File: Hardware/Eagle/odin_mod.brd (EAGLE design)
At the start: 21.4 x 22.8 mm, 36 parts

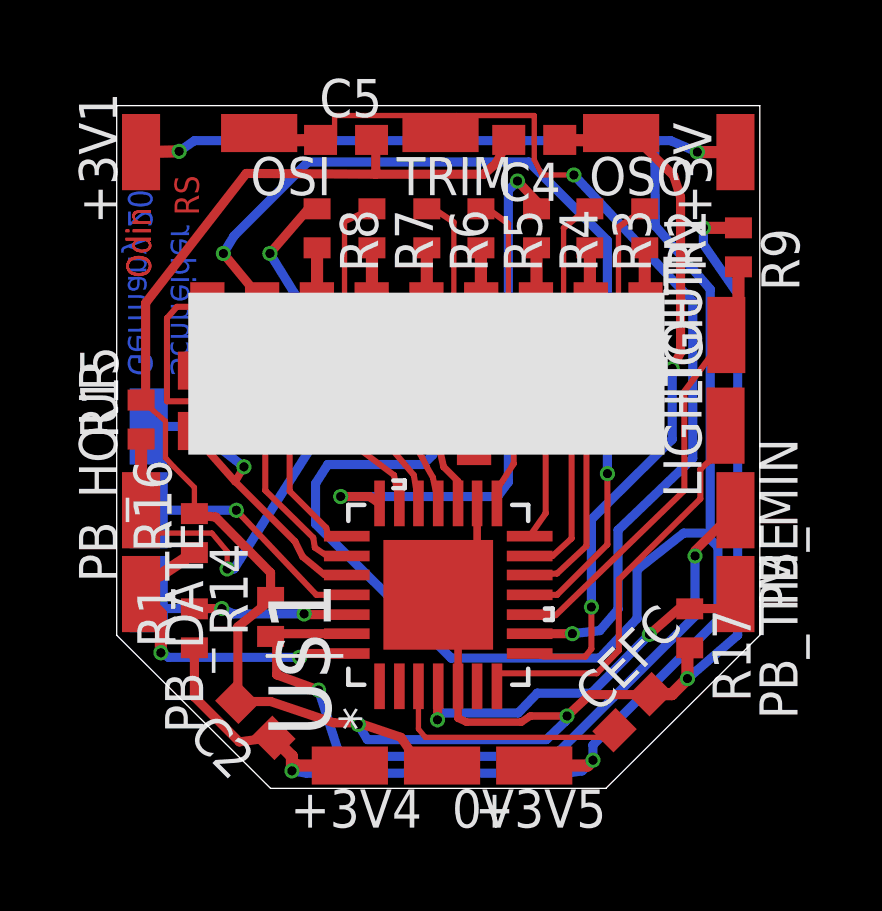
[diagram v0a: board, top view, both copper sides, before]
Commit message: Reviewed Odin module.
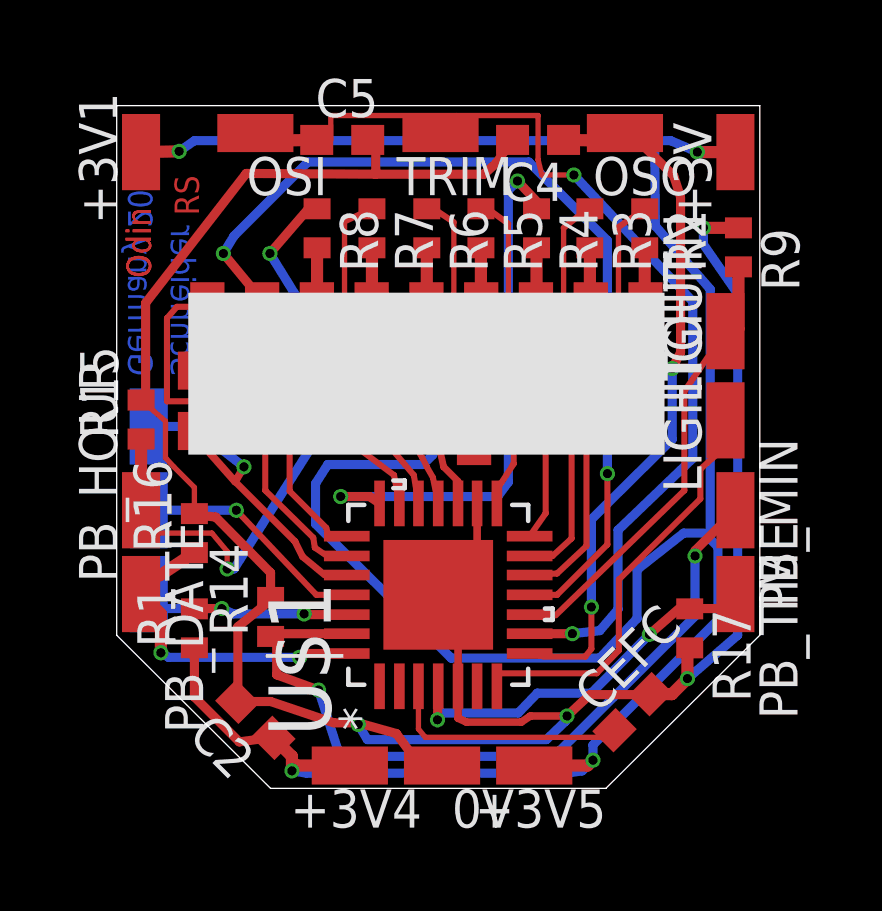
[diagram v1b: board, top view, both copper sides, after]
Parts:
- moved LIGHTOUT 0.18 mm to (20.2, 12.3)
- moved LIGHTIN 0.13 mm to (20.2, 15.2)
- moved C4 0.13 mm to (14.0, 21.6)
- moved C5 0.13 mm to (7.47, 21.6)
- moved OSI 0.13 mm to (4.57, 21.8)
- moved OSO 0.13 mm to (16.9, 21.8)
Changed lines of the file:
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@@
 <element name="R14" library="resistor" package="R0402" value="4.7k" x="5.08" y="5.715" rot="R90"/>
 <element name="R15" library="resistor" package="R0402" value="4.7k" x="0.762" y="12.2936" rot="R90"/>
-<element name="C4" library="resistor" package="C0603" value="12 pF" x="13.8684" y="21.6154" rot="R180"/>
-<element name="C5" library="resistor" package="C0603" value="12 pF" x="7.5946" y="21.6154"/>
+<element name="C4" library="resistor" package="C0603" value="12 pF" x="13.9954" y="21.6154" rot="R180"/>
+<element name="C5" library="resistor" package="C0603" value="12 pF" x="7.4676" y="21.6154"/>
 <element name="U$3" library="pulsar_p3_display" package="PULSAR_P3_LED_DISPLAY" value="PULSAR_P3_DISPLAY" x="2.3368" y="11.1252"/>
 <element name="+3V" library="wirepad" package="SMD1,27-2,54" value="2" x="20.574" y="21.209"/>
@@
 <element name="PAD2" library="wirepad" package="SMD1,27-2,54" value="1" x="1.016" y="9.271" rot="MR0"/>
 <element name="PAD5" library="wirepad" package="SMD1,27-2,54" value="1" x="1.016" y="6.477" rot="MR0"/>
-<element name="OSI" library="wirepad" package="SMD1,27-2,54" value="1" x="4.699" y="21.844" rot="R90"/>
-<element name="OSO" library="wirepad" package="SMD1,27-2,54" value="1" x="16.764" y="21.844" rot="R90"/>
+<element name="OSI" library="wirepad" package="SMD1,27-2,54" value="1" x="4.572" y="21.844" rot="R90"/>
+<element name="OSO" library="wirepad" package="SMD1,27-2,54" value="1" x="16.891" y="21.844" rot="R90"/>
 <element name="+3V4" library="wirepad" package="SMD1,27-2,54" value="1" x="7.7216" y="0.762" rot="R90"/>
 <element name="+3V5" library="wirepad" package="SMD1,27-2,54" value="1" x="13.8684" y="0.762" rot="R90"/>
-<element name="LIGHTIN" library="wirepad" package="SMD1,27-2,54" value="1" x="20.2692" y="15.113"/>
-<element name="LIGHTOUT" library="wirepad" package="SMD1,27-2,54" value="1" x="20.2438" y="12.0904"/>
+<element name="LIGHTIN" library="wirepad" package="SMD1,27-2,54" value="1" x="20.2438" y="15.24"/>
+<element name="LIGHTOUT" library="wirepad" package="SMD1,27-2,54" value="1" x="20.2438" y="12.2682"/>
 <element name="TRIM" library="wirepad" package="SMD1,27-2,54" value="1" x="10.7442" y="21.844" rot="R90"/>
 <element name="R9" library="resistor" package="R0402" value="47k" x="20.6756" y="18.034" rot="R270"/>
@@
 <wire x1="4.2672" y1="20.4978" x2="8.5852" y2="20.4724" width="0.3048" layer="1"/>
 <wire x1="0.9144" y1="13.0302" x2="0.9144" y2="16.1798" width="0.3048" layer="1"/>
-<wire x1="8.7884" y1="21.5646" x2="8.4446" y2="21.6154" width="0.1524" layer="1"/>
+<wire x1="8.7884" y1="21.5646" x2="8.3176" y2="21.6154" width="0.1524" layer="1"/>
 <wire x1="0.9144" y1="13.0302" x2="0.762" y2="12.9436" width="0.1524" layer="1"/>
 <wire x1="3.2512" y1="9.0424" x2="5.08" y2="7.1882" width="0.3048" layer="1"/>
@@
 <wire x1="2.5908" y1="9.1186" x2="2.54" y2="9.159" width="0.1524" layer="1"/>
 <wire x1="10.0584" y1="0.762" x2="10.795" y2="0.762" width="0.3048" layer="1"/>
-<wire x1="9.4234" y1="1.7018" x2="10.0584" y2="0.762" width="0.3048" layer="1"/>
+<wire x1="9.271" y1="1.8288" x2="10.0584" y2="0.762" width="0.3048" layer="1"/>
 <wire x1="7.1882" y1="2.1844" x2="8.001" y2="2.1844" width="0.3048" layer="1"/>
-<wire x1="8.001" y1="2.1844" x2="9.4234" y2="1.7018" width="0.3048" layer="1"/>
+<wire x1="8.001" y1="2.1844" x2="9.271" y2="1.8288" width="0.3048" layer="1"/>
 <wire x1="5.08" y1="2.8956" x2="7.1882" y2="2.1844" width="0.3048" layer="1"/>
 <wire x1="4.064" y1="2.8956" x2="5.08" y2="2.8956" width="0.3048" layer="1"/>
@@
 <wire x1="8.5852" y1="20.4724" x2="12.192" y2="20.4724" width="0.3048" layer="1"/>
 <wire x1="12.192" y1="20.4724" x2="12.5984" y2="20.8398" width="0.3048" layer="1"/>
-<wire x1="12.5984" y1="20.8398" x2="13.0184" y2="21.6154" width="0.3048" layer="1"/>
+<wire x1="12.5984" y1="20.8398" x2="13.1454" y2="21.6154" width="0.3048" layer="1"/>
 <contactref element="R9" pad="1"/>
 <wire x1="20.4216" y1="18.669" x2="20.701" y2="18.669" width="0.1524" layer="1"/>
@@
 <contactref element="C4" pad="1"/>
 <contactref element="OSO" pad="1"/>
-<wire x1="16.764" y1="21.844" x2="16.51" y2="21.59" width="0.1524" layer="1"/>
+<wire x1="16.891" y1="21.844" x2="16.51" y2="21.59" width="0.1524" layer="1"/>
 <wire x1="15.7734" y1="4.6482" x2="15.5702" y2="4.3942" width="0.2032" layer="1"/>
 <wire x1="15.7734" y1="6.0452" x2="15.7734" y2="4.6482" width="0.2032" layer="1"/>
@@
 <wire x1="18.4658" y1="13.9954" x2="18.4658" y2="11.6332" width="0.3048" layer="16"/>
 <wire x1="16.8148" y1="22.098" x2="18.5166" y2="20.4216" width="0.3048" layer="1"/>
-<wire x1="16.8148" y1="22.098" x2="16.764" y2="21.844" width="0.1524" layer="1"/>
+<wire x1="16.8148" y1="22.098" x2="16.891" y2="21.844" width="0.1524" layer="1"/>
 <via x="15.7734" y="6.0452" extent="1-16" drill="0.3048"/>
 <via x="18.4658" y="13.9954" extent="1-16" drill="0.3048"/>
 <wire x1="15.5702" y1="4.3942" x2="14.1732" y2="4.3942" width="0.2032" layer="1"/>
 <wire x1="14.1732" y1="4.3942" x2="13.716" y2="4.4958" width="0.1778" layer="1"/>
-<wire x1="16.51" y1="21.59" x2="14.7184" y2="21.6154" width="0.4064" layer="1"/>
+<wire x1="16.51" y1="21.59" x2="14.8454" y2="21.6154" width="0.4064" layer="1"/>
 <wire x1="18.4658" y1="13.9954" x2="18.7452" y2="14.5288" width="0.3048" layer="1"/>
 <wire x1="18.7452" y1="14.5288" x2="18.7452" y2="19.7104" width="0.3048" layer="1"/>
@@
 <contactref element="C5" pad="1"/>
 <contactref element="OSI" pad="1"/>
-<wire x1="4.699" y1="21.844" x2="4.953" y2="21.59" width="0.1524" layer="1"/>
+<wire x1="4.572" y1="21.844" x2="4.953" y2="21.59" width="0.1524" layer="1"/>
 <wire x1="15.1384" y1="5.1562" x2="13.716" y2="5.1562" width="0.3048" layer="1"/>
 <wire x1="16.0528" y1="5.2578" x2="15.1384" y2="5.1562" width="0.3048" layer="16"/>
@@
 <wire x1="15.1892" y1="20.447" x2="19.1516" y2="16.2306" width="0.3048" layer="16"/>
 <wire x1="14.1224" y1="20.447" x2="15.1892" y2="20.447" width="0.1778" layer="1"/>
-<wire x1="13.8684" y1="20.955" x2="14.1224" y2="20.447" width="0.1778" layer="1"/>
-<wire x1="13.8684" y1="22.4282" x2="13.8684" y2="20.955" width="0.1778" layer="1"/>
-<wire x1="7.2136" y1="22.4282" x2="11.2776" y2="22.4282" width="0.1778" layer="1"/>
-<wire x1="7.2136" y1="21.6154" x2="7.2136" y2="22.4282" width="0.1778" layer="1"/>
-<wire x1="7.2136" y1="21.6154" x2="6.7446" y2="21.6154" width="0.1524" layer="1"/>
+<wire x1="13.9954" y1="20.955" x2="14.1224" y2="20.447" width="0.1778" layer="1"/>
+<wire x1="13.9954" y1="22.4282" x2="13.9954" y2="20.955" width="0.1778" layer="1"/>
+<wire x1="7.0866" y1="22.4282" x2="11.2776" y2="22.4282" width="0.1778" layer="1"/>
+<wire x1="7.0866" y1="21.6154" x2="7.0866" y2="22.4282" width="0.1778" layer="1"/>
+<wire x1="7.0866" y1="21.6154" x2="6.6176" y2="21.6154" width="0.1524" layer="1"/>
 <via x="15.1384" y="5.1562" extent="1-16" drill="0.3048"/>
 <via x="15.1892" y="20.447" extent="1-16" drill="0.3048"/>
 <contactref element="TRIM" pad="1"/>
-<wire x1="13.8684" y1="22.4282" x2="11.2776" y2="22.4282" width="0.1778" layer="1"/>
+<wire x1="13.9954" y1="22.4282" x2="11.2776" y2="22.4282" width="0.1778" layer="1"/>
 <wire x1="11.2776" y1="22.4282" x2="10.7442" y2="21.844" width="0.1524" layer="1"/>
-<wire x1="4.953" y1="21.59" x2="6.7446" y2="21.6154" width="0.4064" layer="1"/>
+<wire x1="4.953" y1="21.59" x2="6.6176" y2="21.6154" width="0.4064" layer="1"/>
 </signal>
 <signal name="RB1/LED_M6">
@@
 <wire x1="18.8722" y1="9.9314" x2="14.5796" y2="5.7658" width="0.2032" layer="1"/>
 <wire x1="18.8722" y1="13.2334" x2="18.8722" y2="9.9314" width="0.2032" layer="1"/>
-<wire x1="20.2692" y1="15.113" x2="18.8722" y2="13.2334" width="0.2032" layer="1"/>
+<wire x1="20.2438" y1="15.24" x2="18.8722" y2="13.2334" width="0.2032" layer="1"/>
 <contactref element="R9" pad="2"/>
-<wire x1="20.2692" y1="15.113" x2="20.701" y2="15.1638" width="0.1524" layer="1"/>
+<wire x1="20.2438" y1="15.24" x2="20.701" y2="15.1638" width="0.1524" layer="1"/>
 <wire x1="20.6756" y1="17.384" x2="20.6756" y2="15.3162" width="0.4064" layer="1"/>
-<wire x1="20.6756" y1="15.3162" x2="20.2692" y2="15.113" width="0.4064" layer="1"/>
+<wire x1="20.6756" y1="15.3162" x2="20.2438" y2="15.24" width="0.4064" layer="1"/>
 </signal>
 <signal name="OSC2/RA6">
@@
 <wire x1="19.4056" y1="9.652" x2="19.4056" y2="10.6426" width="0.2032" layer="1"/>
 <wire x1="19.4056" y1="10.6426" x2="20.574" y2="11.684" width="0.2032" layer="1"/>
-<wire x1="20.574" y1="11.684" x2="20.2438" y2="12.0904" width="0.1524" layer="1"/>
+<wire x1="20.574" y1="11.684" x2="20.2438" y2="12.2682" width="0.1524" layer="1"/>
 </signal>
 <signal name="RA5/SW4">

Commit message: Optimizations.
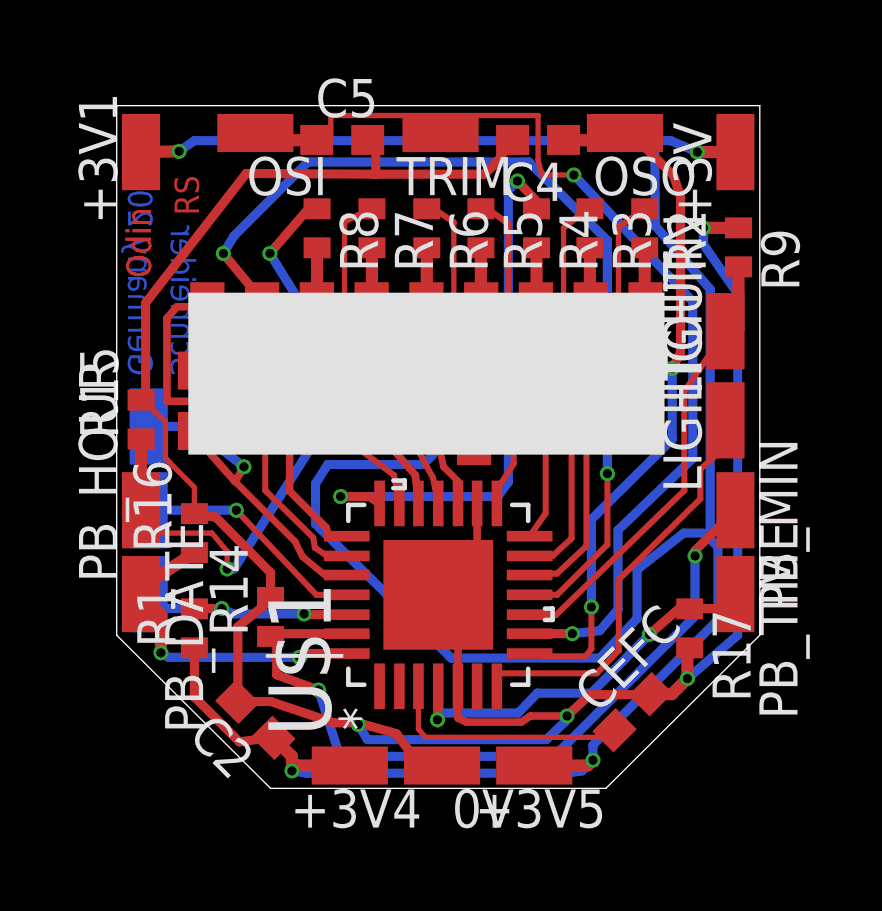
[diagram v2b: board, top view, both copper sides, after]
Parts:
- R9: value 47k -> 68k
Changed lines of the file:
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@@
 <element name="LIGHTOUT" library="wirepad" package="SMD1,27-2,54" value="1" x="20.2438" y="12.2682"/>
 <element name="TRIM" library="wirepad" package="SMD1,27-2,54" value="1" x="10.7442" y="21.844" rot="R90"/>
-<element name="R9" library="resistor" package="R0402" value="47k" x="20.6756" y="18.034" rot="R270"/>
+<element name="R9" library="resistor" package="R0402" value="68k" x="20.6756" y="18.034" rot="R270"/>
 </elements>
 <signals>
@@
 <contactref element="U$1" pad="22"/>
 <contactref element="U$3" pad="P$9_KATHODE_10_MIN"/>
-<wire x1="7.62" y1="8.4074" x2="7.0104" y2="8.4074" width="0.2032" layer="1"/>
-<wire x1="1.6256" y1="12.9032" x2="1.6256" y2="15.6718" width="0.2032" layer="1"/>
-<wire x1="7.0104" y1="8.4074" x2="6.9342" y2="8.6868" width="0.2032" layer="1"/>
-<wire x1="6.9342" y1="8.6868" x2="5.715" y2="9.906" width="0.2032" layer="1"/>
-<wire x1="5.715" y1="9.906" x2="5.715" y2="12.4206" width="0.2032" layer="1"/>
-<wire x1="1.6256" y1="12.9032" x2="5.0546" y2="12.9032" width="0.2032" layer="1"/>
-<wire x1="5.0546" y1="12.9032" x2="5.715" y2="12.4206" width="0.2032" layer="1"/>
-<wire x1="1.6256" y1="15.6718" x2="1.9558" y2="16.0528" width="0.2032" layer="1"/>
-<wire x1="1.9558" y1="16.0528" x2="2.96545" y2="16.0528" width="0.2032" layer="1"/>
+<wire x1="7.62" y1="8.4074" x2="7.0104" y2="8.4074" width="0.254" layer="1"/>
+<wire x1="1.6256" y1="12.9032" x2="1.6256" y2="15.6718" width="0.254" layer="1"/>
+<wire x1="7.0104" y1="8.4074" x2="6.9342" y2="8.6868" width="0.254" layer="1"/>
+<wire x1="6.9342" y1="8.6868" x2="5.715" y2="9.906" width="0.254" layer="1"/>
+<wire x1="5.715" y1="9.906" x2="5.715" y2="12.4206" width="0.254" layer="1"/>
+<wire x1="1.6256" y1="12.9032" x2="5.0546" y2="12.9032" width="0.254" layer="1"/>
+<wire x1="5.0546" y1="12.9032" x2="5.715" y2="12.4206" width="0.254" layer="1"/>
+<wire x1="1.6256" y1="15.6718" x2="1.9558" y2="16.0528" width="0.254" layer="1"/>
+<wire x1="1.9558" y1="16.0528" x2="2.96545" y2="16.0528" width="0.254" layer="1"/>
 <wire x1="2.96545" y1="16.0528" x2="2.9718" y2="16.04645" width="0.1524" layer="1"/>
 </signal>
@@
 <contactref element="U$1" pad="19"/>
 <contactref element="U$3" pad="P$10_KATHODE_1_HOUR"/>
-<wire x1="9.8552" y1="10.4394" x2="7.2136" y2="13.5636" width="0.2032" layer="1"/>
-<wire x1="10.0076" y1="9.4996" x2="9.8552" y2="10.4394" width="0.2032" layer="1"/>
-<wire x1="7.2136" y1="13.5636" x2="3.683" y2="13.5636" width="0.2032" layer="1"/>
+<wire x1="9.906" y1="10.4394" x2="7.2136" y2="13.5636" width="0.254" layer="1"/>
+<wire x1="10.0076" y1="9.4996" x2="9.906" y2="10.4394" width="0.254" layer="1"/>
+<wire x1="7.2136" y1="13.5636" x2="3.683" y2="13.5636" width="0.254" layer="1"/>
 <wire x1="3.683" y1="13.5636" x2="2.81305" y2="13.92555" width="0.2032" layer="1"/>
 </signal>
